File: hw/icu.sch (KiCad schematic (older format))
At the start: 4 parts, among them J101 AMPSEAL_8_POS_VERT_BLACK_SEAL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, J102 AMPSEAL_23_POS_VERT_GRAY_SEAL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

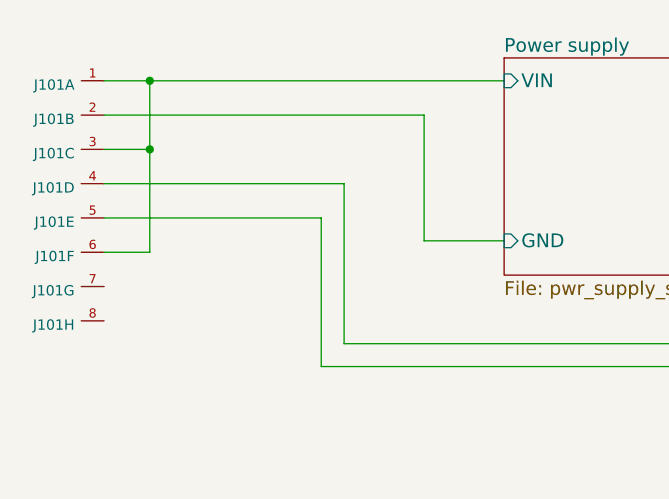
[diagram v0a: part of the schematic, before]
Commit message: implementing icu in CM_6.2.1
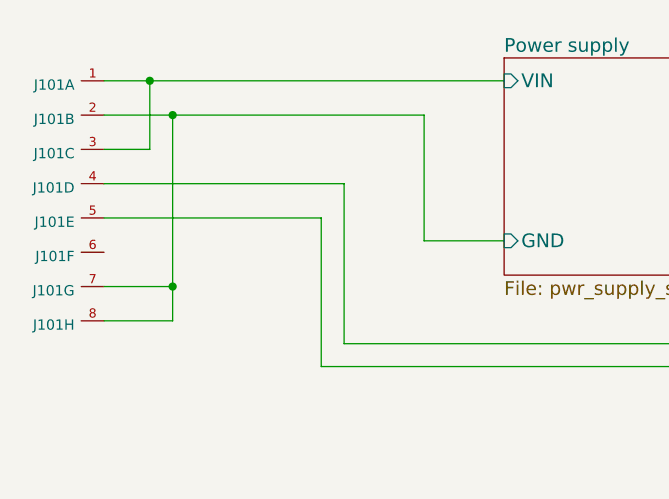
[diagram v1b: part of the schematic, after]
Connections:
- net Power supply/GND: now also J101.7 (S), J101.8 (S)
- net Power supply/VIN: no longer J101.6 (S)
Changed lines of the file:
@@
 Connection ~ 1650 2100
 Wire Wire Line
-	1650 2850 1450 2850
-Connection ~ 1650 2400
-Wire Wire Line
-	1450 2250 2850 2250
+	1450 2250 1750 2250
 Wire Wire Line
 	2850 2250 2850 2800
@@
 Wire Wire Line
 	1650 2100 3200 2100
-Wire Wire Line
-	1650 2400 1650 2850
 $Comp
 L icu-rescue:VDD #PWR0101
@@
 Wire Wire Line
 	7200 5750 5950 5750
+Wire Wire Line
+	1450 3000 1750 3000
+Wire Wire Line
+	1750 3000 1750 2250
+Connection ~ 1750 2250
+Wire Wire Line
+	1750 2250 2850 2250
+Wire Wire Line
+	1750 3000 1750 3150
+Wire Wire Line
+	1750 3150 1450 3150
+Connection ~ 1750 3000
 $EndSCHEMATC
